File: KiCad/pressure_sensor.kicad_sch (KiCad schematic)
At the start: 9 parts, among them IC3 MS5849-30BA, U14 SN74LV1T34DCK, U7 SN74LV1T34DCK, U8 PCA9306

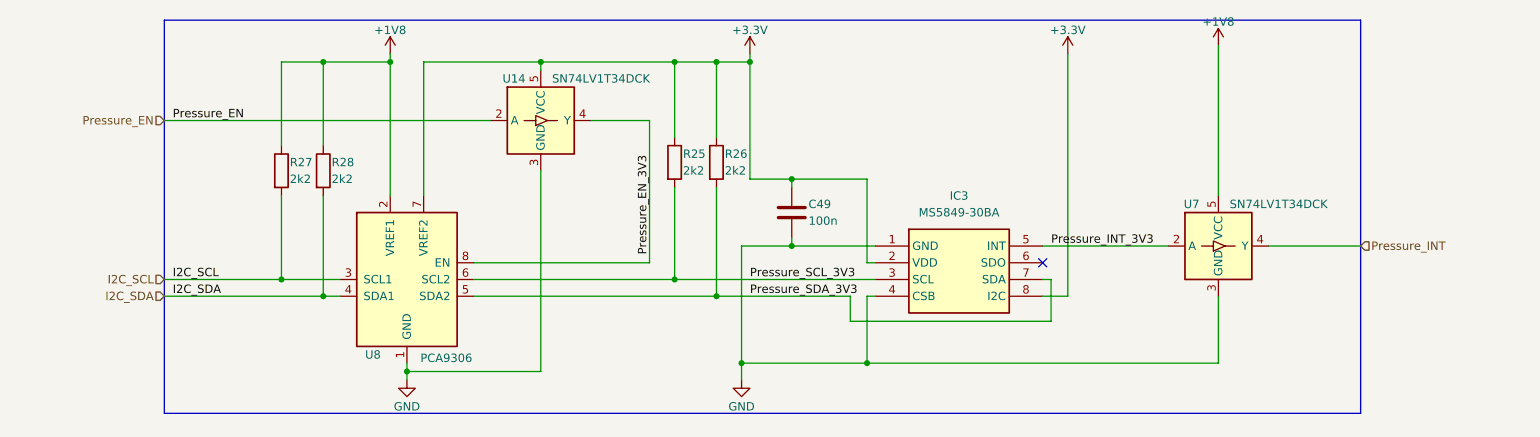
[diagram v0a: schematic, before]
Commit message: Added some TODOs, fixed some TODOs
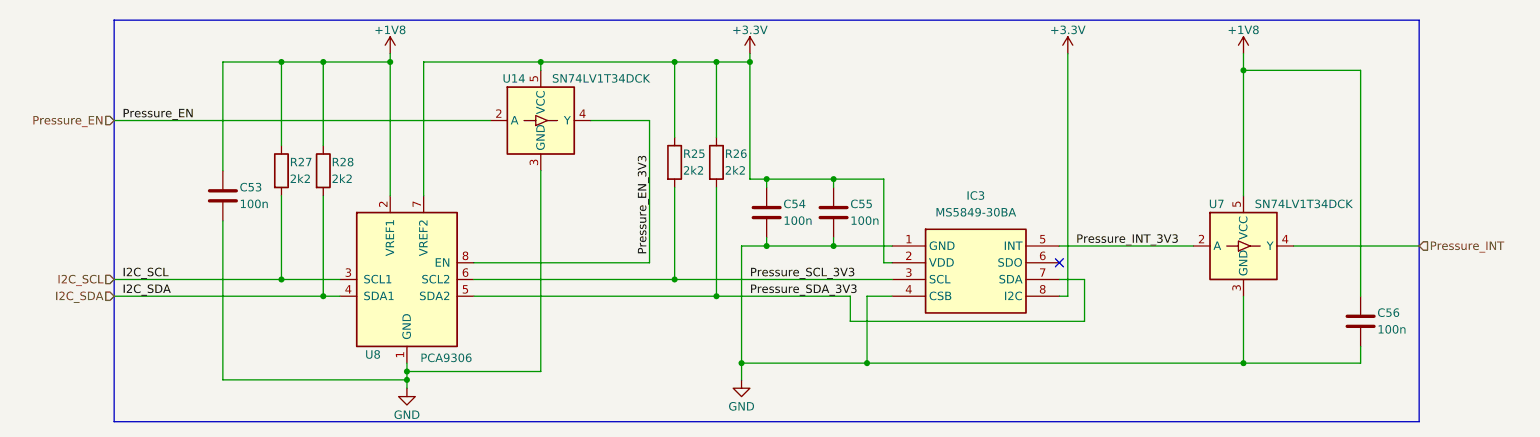
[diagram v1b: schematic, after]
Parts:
- added C53, C54, C56: 100n, Capacitor_SMD:C_0402_1005Metric, symbol Device:C
- renumbered C49 to C55
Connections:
- net +1V8: now also C53.1, C56.1
- net +3.3V: now also C54.1
- net GND: now also C53.2, C54.2, C56.2
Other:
- moved on the sheet: C55, IC3, U7
